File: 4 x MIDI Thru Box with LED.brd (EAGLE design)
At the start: 84.8 x 86.3 mm, 25 parts, among them IC1 7805, IC2 74AC14N, J1 xx amps, X1 MIDI, X2 MIDI, X3 MIDI, X4 MIDI, X5 MIDI

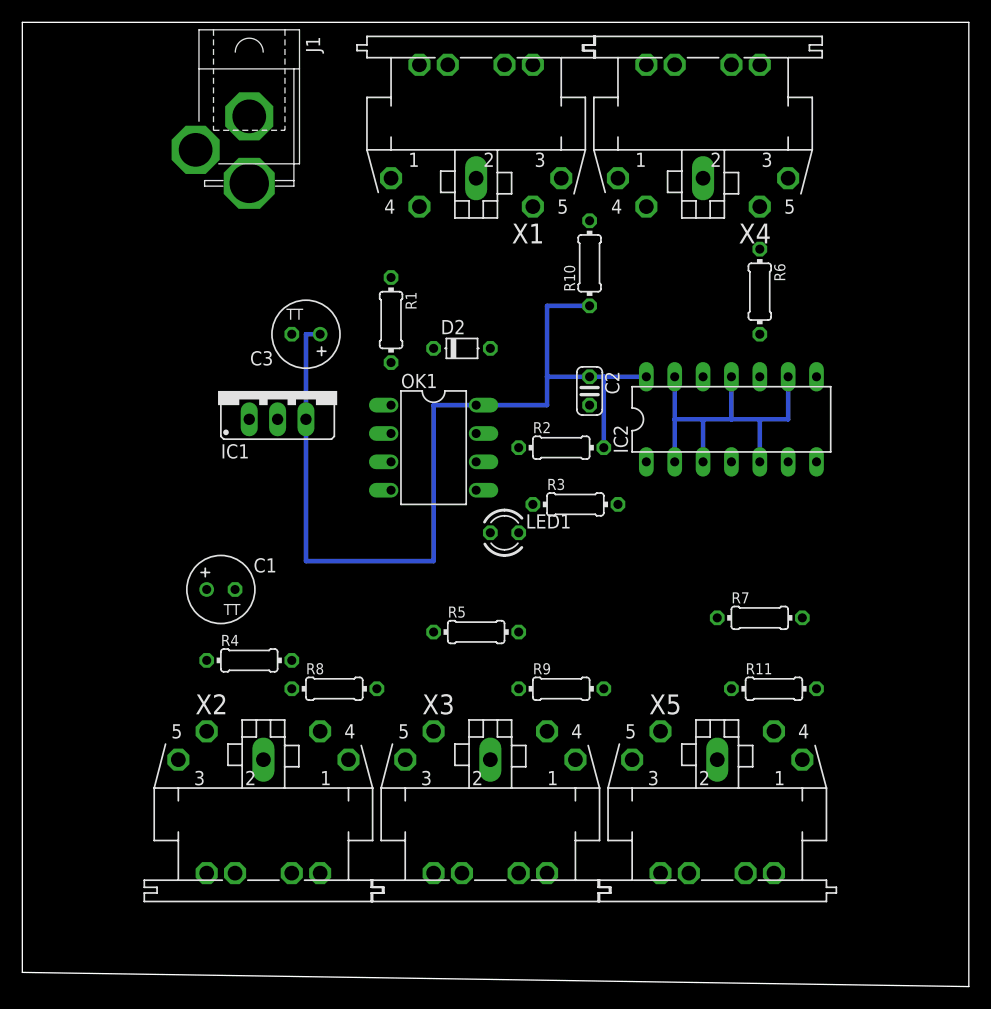
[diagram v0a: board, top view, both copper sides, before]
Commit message: Completed PCB design
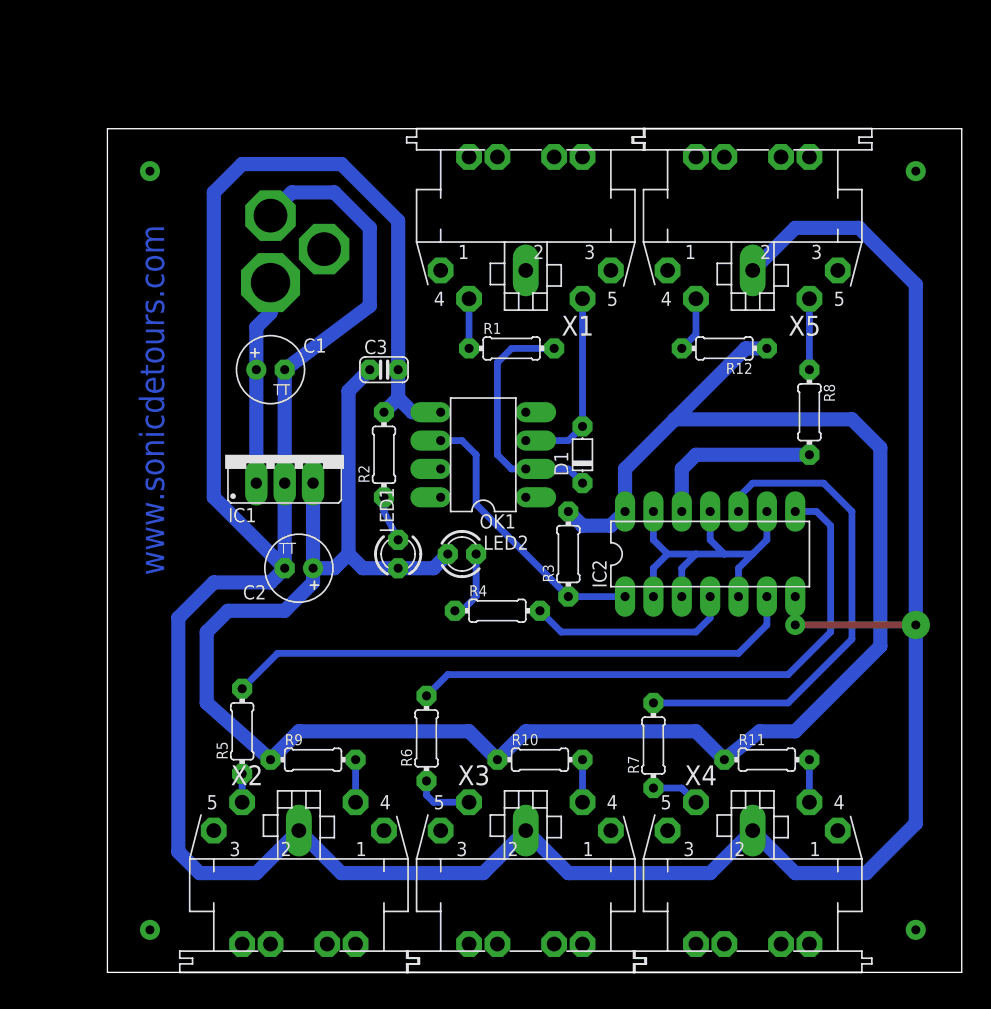
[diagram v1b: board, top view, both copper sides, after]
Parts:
- removed D2: 1N4148, diode:D-5
- added D1: 1N4148, diode:D-5
- added LED2: Red, led:LED3MM
- added R12: 220, rcl:0204/7
- C2: value 100nF -> 0.1uF; device rcl:C025-024X044 -> rcl:TT2D6
- C3: value 0.1uF -> 100nF; device rcl:TT2D6 -> rcl:C025-024X044
- LED1: value (none) -> Green
- R2: value 820 -> 330
- R3: value 330 -> 820
- R4: value 220 -> 330
- moved X4 73.8 mm to (57.8, 5.08), turned to 0 degrees
- moved X5 59.1 mm to (57.8, 70.5), turned to 180 degrees
- moved R6 49.9 mm to (28.6, 21.0), turned to 90 degrees
- moved R8 49.2 mm to (62.9, 50.2), turned to 270 degrees
- moved R10 44.7 mm to (38.7, 19.1), turned to 0 degrees
- moved C2 30.5 mm to (17.1, 36.2), turned to 180 degrees
- moved R9 23.1 mm to (18.4, 19.1)
- moved R5 22.8 mm to (12.1, 21.6), turned to 90 degrees
- moved R4 22.7 mm to (34.9, 32.4)
- moved C1 20.2 mm to (14.6, 54.0)
- moved R2 15.9 mm to (24.8, 46.4), turned to 90 degrees
- moved R7 14.9 mm to (48.9, 20.3), turned to 90 degrees
- moved IC2 12.2 mm to (54.0, 37.5)
- moved R1 11.1 mm to (36.2, 55.9), turned to 0 degrees
- moved LED1 9.71 mm to (26.0, 37.5), turned to 90 degrees
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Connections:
- removed net N$8: C1.+, IC1.IN
- new net N$6: C1.+, IC1.IN, J1.3
- new net N$9: LED1.K, R2.1
- net +5V: now also C2.+, C3.1, LED2.A, R12.1, R3.2; no longer C2.1, C3.+, R2.2, R8.1
- net GND: now also C2.-, C3.2, R2.2; no longer C2.2, C3.-
- net MIDI_IN: now also R3.1; no longer R2.1
- net N$1: now also R5.2; no longer R4.2
- net N$11: now also D1.A; no longer D2.A
- net N$14: now also D1.C; no longer D2.C
- net N$2: now also R7.2; no longer R6.2
- net N$21: now also R7.1; no longer R6.1
- net N$22: now also R6.2; no longer R5.2
- net N$23: now also R5.1; no longer R4.1
- net N$26: now also R8.2; no longer R7.2
- net N$3: now also R8.1; no longer R7.1
- net N$4: now also R9.2; no longer R8.2
- net N$41: now also R6.1; no longer R5.1
- net N$5: now also LED2.K, R4.1; no longer LED1.K, R3.1
- net N$52: now also R12.2; no longer R11.2
- net N$53: now also R11.2; no longer R10.2
- net N$54: now also R10.2; no longer R9.2
- net N$65: now also R4.2; no longer R3.2
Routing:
- net GND: track 0.00 -> 313.8 mm, vias 0 -> 2
- net +5V: track 85.1 -> 192.4 mm
- net N$1: track 0.00 -> 51.9 mm
- net N$22: track 0.00 -> 51.8 mm
- net N$2: track 0.00 -> 44.6 mm
- net MIDI_IN: track 0.00 -> 24.9 mm
- net N$14: track 0.00 -> 22.5 mm
- net N$11: track 0.00 -> 19.6 mm
- net N$6: track 0.00 -> 18.5 mm
- net N$65: track 0.00 -> 18.5 mm
- net N$26: track 0.00 -> 15.8 mm
- net N$3: track 0.00 -> 6.35 mm
- net N$5: track 0.00 -> 6.24 mm
- net N$41: track 0.00 -> 5.34 mm
- net N$52: track 0.00 -> 4.97 mm
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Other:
- board size 84.8 x 86.3 mm -> 76.5 x 75.6 mm
- board text added: "www.sonicdetours.com"

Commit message: Version 1.0
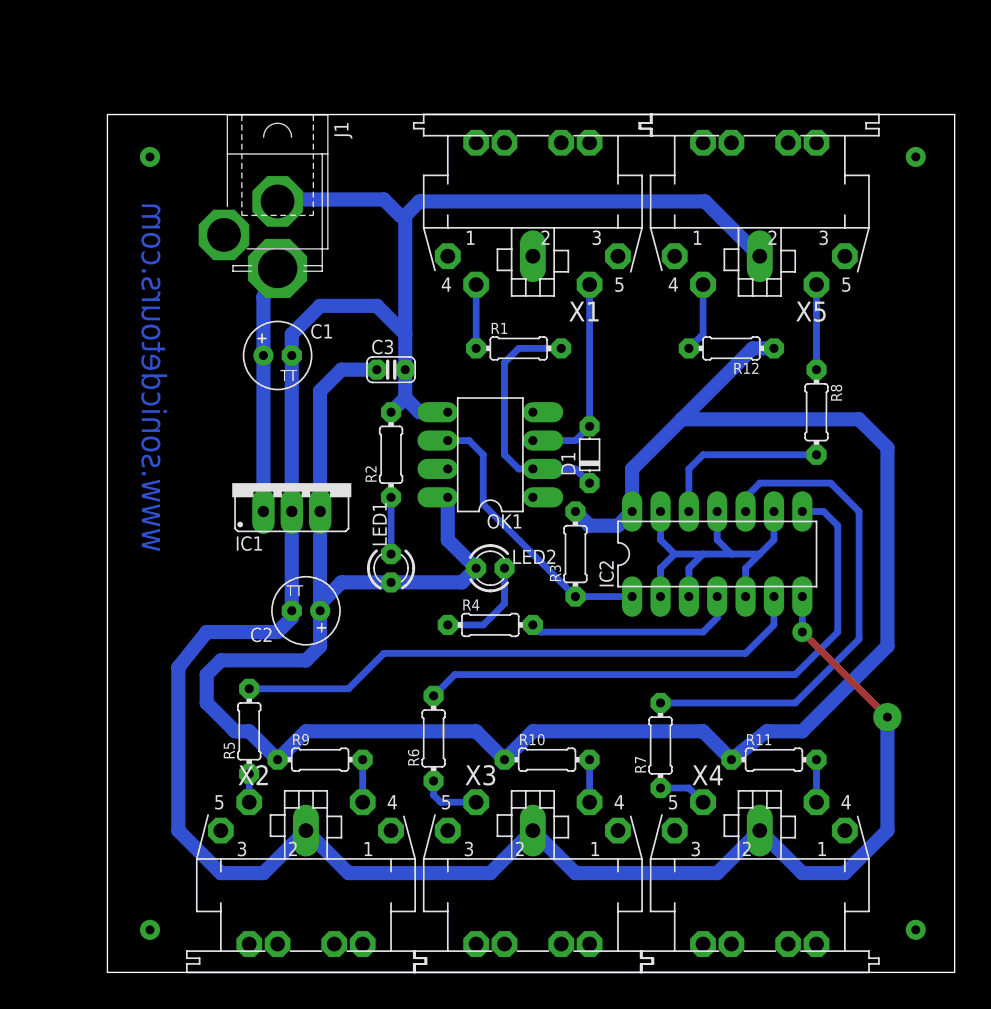
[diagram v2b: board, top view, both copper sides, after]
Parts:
- J1: value xx amps -> 9V DC
- LED1: value Green -> Power
- LED2: value Red -> Midi In
- moved C2 3.86 mm to (17.8, 32.4)
- moved LED2 2.84 mm to (34.3, 36.2)
- moved IC1 2.62 mm to (16.5, 43.8)
- moved LED1 1.42 mm to (25.4, 36.2)
- moved R4 1.42 mm to (34.3, 31.1)
- moved X5 1.42 mm to (58.4, 71.8)
- moved C1 1.42 mm to (15.2, 55.2)
- moved J1 1.42 mm to (15.2, 68.6), flipped to the top
- moved X1 1.42 mm to (38.1, 71.8)
- moved R12 0.64 mm to (55.9, 55.9)
- moved X4 0.64 mm to (58.4, 5.08)
- moved R6 0.64 mm to (29.2, 21.0)
- moved R9 0.64 mm to (19.1, 19.1)
- moved X2 0.64 mm to (17.8, 5.08)
- moved R5 0.63 mm to (12.7, 21.6)
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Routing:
- net GND: track 313.8 -> 233.6 mm
- net +5V: track 192.4 -> 200.2 mm
- net N$6: track 18.5 -> 22.1 mm
- net N$5: track 6.24 -> 9.04 mm
- net N$52: track 4.97 -> 6.24 mm
- net N$7: track 4.45 -> 5.71 mm
- net N$3: track 6.35 -> 7.62 mm
- net N$11: track 19.6 -> 20.8 mm
- net N$9: track 4.11 -> 5.08 mm
- net N$65: track 18.5 -> 19.2 mm
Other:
- board size 76.5 x 75.6 mm -> 75.9 x 76.8 mm
